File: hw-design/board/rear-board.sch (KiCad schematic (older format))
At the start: 20 parts, among them J1 CC_INPUT, J2 CC_OUTPUT, P7 CONN_01X16, P8 USB_OTG, P9 CONN_01X16, Q7 2N7002, Q8 2N7002, Q9 IRFML8244TRPBF

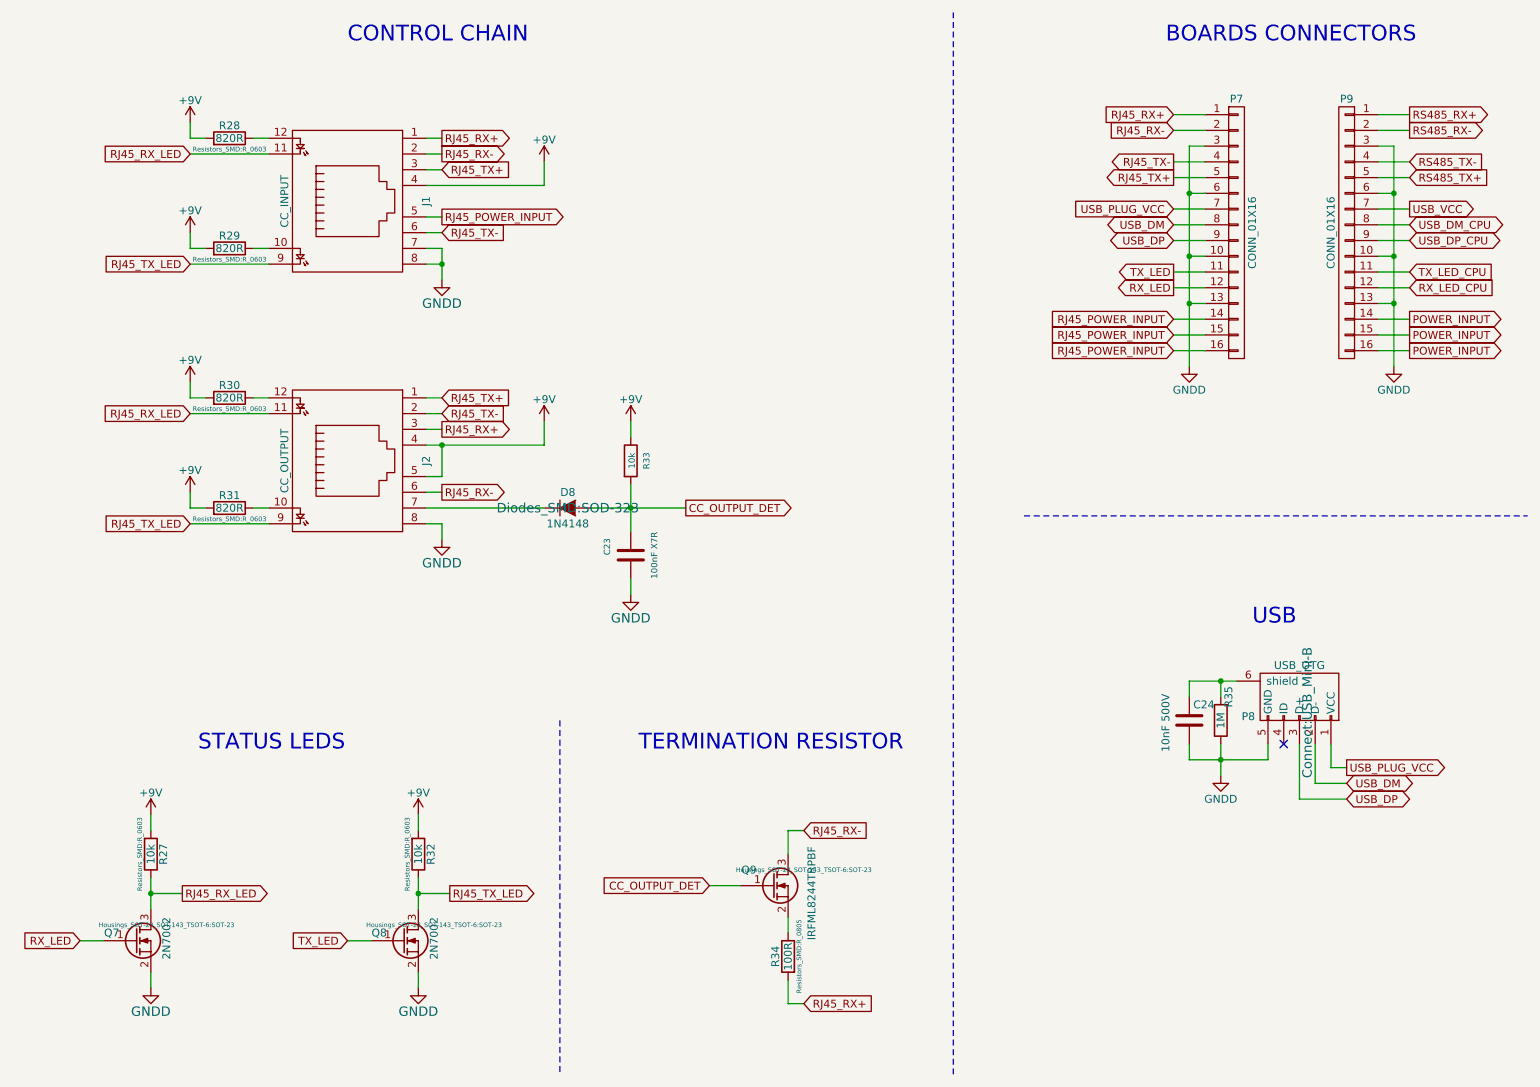
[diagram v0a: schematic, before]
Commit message: fix power voltage
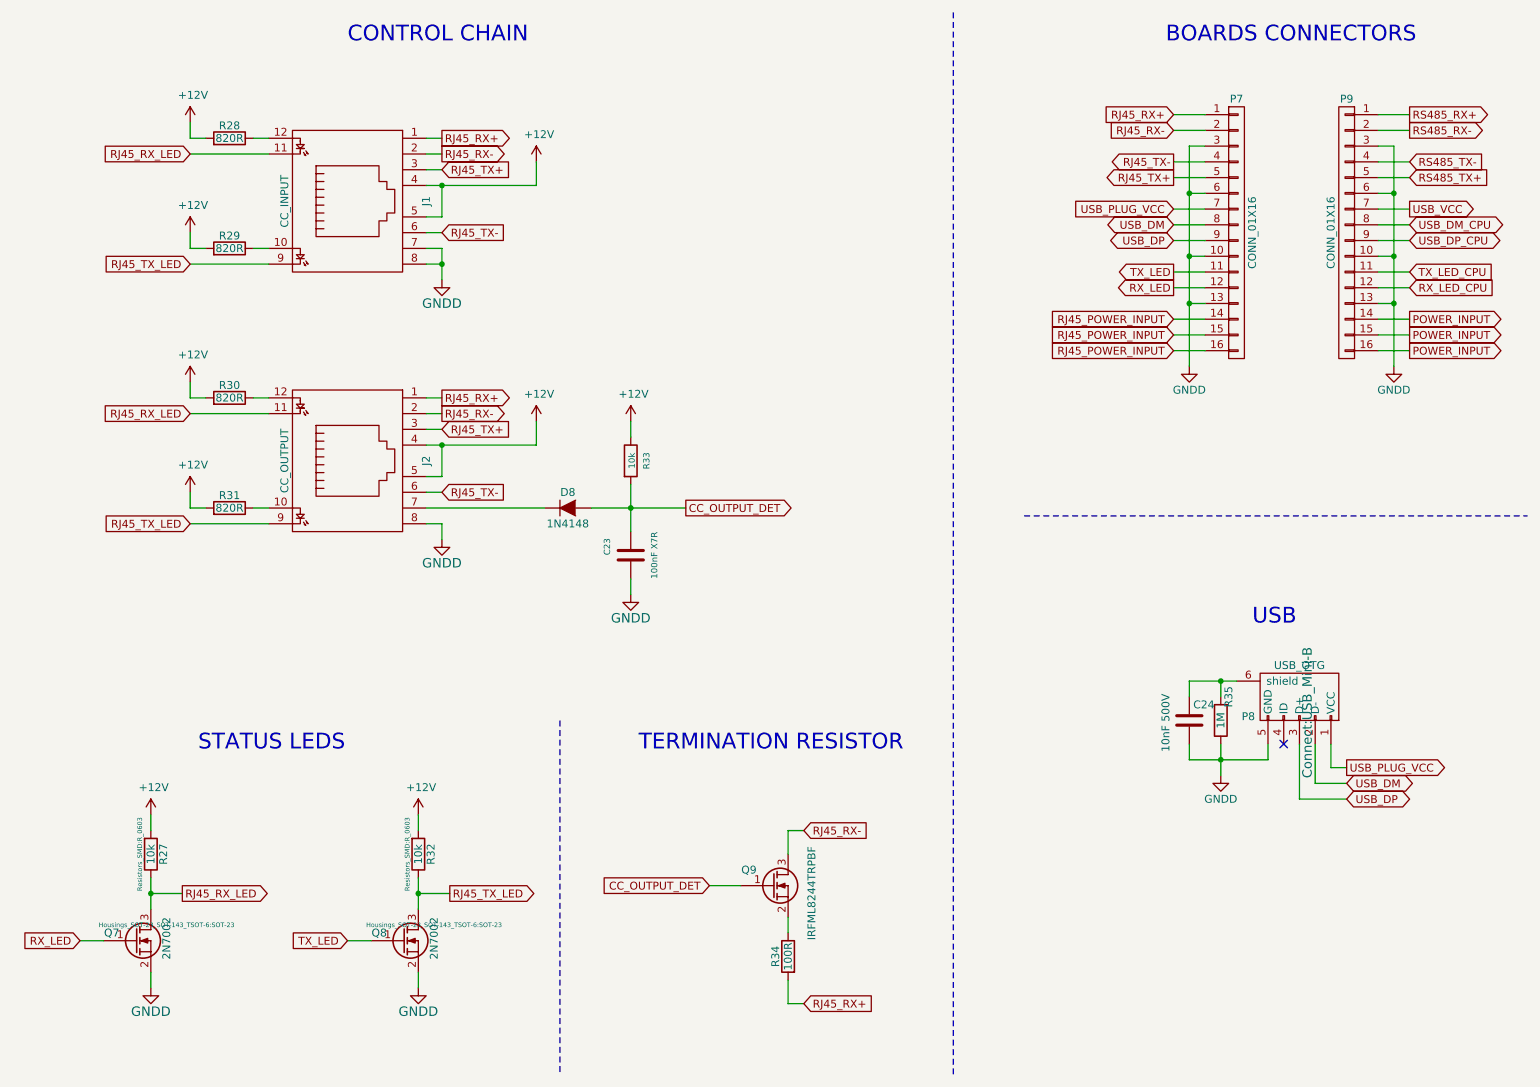
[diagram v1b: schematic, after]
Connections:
- net RJ45_POWER_INPUT: no longer J1.5
- net RJ45_RX+: now also J2.1; no longer J2.3
- net RJ45_RX-: now also J2.2; no longer J2.6
- net RJ45_TX+: now also J2.3; no longer J2.1
- net RJ45_TX-: now also J2.6; no longer J2.2
- net +9V renamed +12V
- net +12V: now also J1.5
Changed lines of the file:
@@
-$EndComp
-$Comp
-L +9V #PWR085
-U 1 1 55B26422
-P 4700 3300
-F 0 "#PWR085" H 4700 3150 50  0001 C CNN
-F 1 "+9V" H 4700 3440 50  0000 C CNN
-F 2 "" H 4700 3300 60  0000 C CNN
-F 3 "" H 4700 3300 60  0000 C CNN
-	1    4700 3300
-	1    0    0    -1
-$EndComp
-$Comp
-L +9V #PWR086
-U 1 1 55B26428
-P 4150 3300
-F 0 "#PWR086" H 4150 3150 50  0001 C CNN
-F 1 "+9V" H 4150 3440 50  0000 C CNN
-F 2 "" H 4150 3300 60  0000 C CNN
-F 3 "" H 4150 3300 60  0000 C CNN
-	1    4150 3300
-	1    0    0    -1
-$EndComp
-$Comp
-L +9V #PWR087
-U 1 1 55B2642E
-P 4150 1650
-F 0 "#PWR087" H 4150 1500 50  0001 C CNN
-F 1 "+9V" H 4150 1790 50  0000 C CNN
-F 2 "" H 4150 1650 60  0000 C CNN
-F 3 "" H 4150 1650 60  0000 C CNN
-	1    4150 1650
-	1    0    0    -1
 $EndComp
 $Comp
@@
 F 0 "D8" H 4300 3950 50  0000 C CNN
 F 1 "1N4148" H 4300 3750 50  0000 C CNN
-F 2 "Diodes_SMD:SOD-323" H 4300 3850 60  0000 C CNN
+F 2 "Diodes_SMD:SOD-323" H 4300 3850 60  0001 C CNN
 F 3 "" H 4300 3850 60  0000 C CNN
 F 4 "1N4148WX-TP" H -250 -250 50  0001 C CNN "MPN"
@@
 F 0 "R30" V 2230 3150 50  0000 C CNN
 F 1 "820R" V 2150 3150 50  0000 C CNN
-F 2 "Resistors_SMD:R_0603" V 2080 3150 30  0000 C CNN
+F 2 "Resistors_SMD:R_0603" V 2080 3150 30  0001 C CNN
 F 3 "" H 2150 3150 30  0000 C CNN
 F 4 "ESR03EZPJ821" H -250 -250 50  0001 C CNN "MPN"
@@
 F 0 "R28" V 2230 1500 50  0000 C CNN
 F 1 "820R" V 2150 1500 50  0000 C CNN
-F 2 "Resistors_SMD:R_0603" V 2080 1500 30  0000 C CNN
+F 2 "Resistors_SMD:R_0603" V 2080 1500 30  0001 C CNN
 F 3 "" H 2150 1500 30  0000 C CNN
 F 4 "ESR03EZPJ821" H -250 -100 50  0001 C CNN "MPN"
@@
 F 0 "R31" V 2230 3850 50  0000 C CNN
 F 1 "820R" V 2150 3850 50  0000 C CNN
-F 2 "Resistors_SMD:R_0603" V 2080 3850 30  0000 C CNN
+F 2 "Resistors_SMD:R_0603" V 2080 3850 30  0001 C CNN
 F 3 "" H 2150 3850 30  0000 C CNN
 F 4 "ESR03EZPJ821" H -250 -250 50  0001 C CNN "MPN"
@@
 F 0 "R29" V 2230 2200 50  0000 C CNN
 F 1 "820R" V 2150 2200 50  0000 C CNN
-F 2 "Resistors_SMD:R_0603" V 2080 2200 30  0000 C CNN
+F 2 "Resistors_SMD:R_0603" V 2080 2200 30  0001 C CNN
 F 3 "" H 2150 2200 30  0000 C CNN
 F 4 "ESR03EZPJ821" H -250 -100 50  0001 C CNN "MPN"
 	1    2150 2200
 	0    1    -1   0
-$EndComp
-$Comp
-L +9V #PWR088
-U 1 1 55B2645C
-P 1900 3050
-F 0 "#PWR088" H 1900 2900 50  0001 C CNN
-F 1 "+9V" H 1900 3190 50  0000 C CNN
-F 2 "" H 1900 3050 60  0000 C CNN
-F 3 "" H 1900 3050 60  0000 C CNN
-	1    1900 3050
-	1    0    0    -1
-$EndComp
-$Comp
-L +9V #PWR089
-U 1 1 55B26462
-P 1900 3750
-F 0 "#PWR089" H 1900 3600 50  0001 C CNN
-F 1 "+9V" H 1900 3890 50  0000 C CNN
-F 2 "" H 1900 3750 60  0000 C CNN
-F 3 "" H 1900 3750 60  0000 C CNN
-	1    1900 3750
-	1    0    0    -1
-$EndComp
-$Comp
-L +9V #PWR090
-U 1 1 55B26468
-P 1900 2100
-F 0 "#PWR090" H 1900 1950 50  0001 C CNN
-F 1 "+9V" H 1900 2240 50  0000 C CNN
-F 2 "" H 1900 2100 60  0000 C CNN
-F 3 "" H 1900 2100 60  0000 C CNN
-	1    1900 2100
-	1    0    0    -1
-$EndComp
-$Comp
-L +9V #PWR091
-U 1 1 55B2646E
-P 1900 1400
-F 0 "#PWR091" H 1900 1250 50  0001 C CNN
-F 1 "+9V" H 1900 1540 50  0000 C CNN
-F 2 "" H 1900 1400 60  0000 C CNN
-F 3 "" H 1900 1400 60  0000 C CNN
-	1    1900 1400
-	1    0    0    -1
 $EndComp
 Text GLabel 3500 1700 2    50   Input ~ 0
@@
 Text GLabel 3500 1600 2    50   Output ~ 0
 RJ45_RX-
-Text GLabel 3500 3150 2    50   Input ~ 0
+Text GLabel 3500 3350 2    50   Input ~ 0
 RJ45_TX+
-Text GLabel 3500 3250 2    50   Input ~ 0
+Text GLabel 3500 3750 2    50   Input ~ 0
 RJ45_TX-
-Text GLabel 3500 3350 2    50   Output ~ 0
+Text GLabel 3500 3150 2    50   Output ~ 0
 RJ45_RX+
-Text GLabel 3500 3750 2    50   Output ~ 0
+Text GLabel 3500 3250 2    50   Output ~ 0
 RJ45_RX-
-Text GLabel 3500 2000 2    50   Output ~ 0
-RJ45_POWER_INPUT
 Text GLabel 5050 3850 2    50   Output ~ 0
 CC_OUTPUT_DET
@@
 $EndComp
 $Comp
-L +9V #PWR094
-U 1 1 55B30E71
-P 1650 5800
-F 0 "#PWR094" H 1650 5650 50  0001 C CNN
-F 1 "+9V" H 1650 5940 50  0000 C CNN
-F 2 "" H 1650 5800 60  0000 C CNN
-F 3 "" H 1650 5800 60  0000 C CNN
-	1    1650 5800
-	1    0    0    -1
-$EndComp
-$Comp
 L Q_NMOS_GSD Q8
 U 1 1 55B30E78
@@
 	1    0    0    1
 $EndComp
-$Comp
-L +9V #PWR096
-U 1 1 55B30E8D
-P 3350 5800
-F 0 "#PWR096" H 3350 5650 50  0001 C CNN
-F 1 "+9V" H 3350 5940 50  0000 C CNN
-F 2 "" H 3350 5800 60  0000 C CNN
-F 3 "" H 3350 5800 60  0000 C CNN
-	1    3350 5800
-	1    0    0    -1
-$EndComp
 Text Notes 1950 5400 0    100  ~ 0
 STATUS LEDS
@@
 F 0 "Q9" H 5500 6350 50  0000 R CNN
 F 1 "IRFML8244TRPBF" V 5850 6500 50  0000 R CNN
-F 2 "Housings_SOT-23_SOT-143_TSOT-6:SOT-23" H 5800 6350 29  0000 C CNN
+F 2 "Housings_SOT-23_SOT-143_TSOT-6:SOT-23" H 5800 6350 29  0001 C CNN
 F 3 "" H 5600 6250 60  0000 C CNN
 F 4 "IRFML8244TRPBF" H -2600 1300 50  0001 C CNN "MPN"
@@
 F 0 "R34" V 5780 6700 50  0000 C CNN
 F 1 "100R" V 5700 6700 50  0000 C CNN
-F 2 "Resistors_SMD:R_0805" V 5630 6700 30  0000 C CNN
+F 2 "Resistors_SMD:R_0805" V 5630 6700 30  0001 C CNN
 F 3 "" H 5700 6700 30  0000 C CNN
 F 4 "ERJ-P06F1000V" H -2600 1300 50  0001 C CNN "MPN"
@@
 	4700 3400 4700 3300
 Wire Wire Line
-	3400 3450 4150 3450
-Wire Wire Line
-	4150 3450 4150 3300
+	3400 3450 4100 3450
 Wire Wire Line
 	3400 3650 3500 3650
@@
 	1900 1500 1900 1400
 Wire Wire Line
-	3400 1800 4150 1800
-Wire Wire Line
-	4150 1800 4150 1650
+	3400 1800 4100 1800
 Connection ~ 3500 2300
 Connection ~ 4700 3850
@@
 Wire Wire Line
 	9450 2850 9650 2850
+$Comp
+L +12V #PWR?
+U 1 1 575F20CD
+P 1900 1400
+F 0 "#PWR?" H 1900 1250 50  0001 C CNN
+F 1 "+12V" H 1918 1574 50  0000 C CNN
+F 2 "" H 1900 1400 60  0000 C CNN
+F 3 "" H 1900 1400 60  0000 C CNN
+	1    1900 1400
+	1    0    0    -1
+$EndComp
+$Comp
+L +12V #PWR?
+U 1 1 575F21C6
+P 1900 2100
+F 0 "#PWR?" H 1900 1950 50  0001 C CNN
+F 1 "+12V" H 1918 2274 50  0000 C CNN
+F 2 "" H 1900 2100 60  0000 C CNN
+F 3 "" H 1900 2100 60  0000 C CNN
+	1    1900 2100
+	1    0    0    -1
+$EndComp
+$Comp
+L +12V #PWR?
+U 1 1 575F2249
+P 4100 1650
+F 0 "#PWR?" H 4100 1500 50  0001 C CNN
+F 1 "+12V" H 4118 1824 50  0000 C CNN
+F 2 "" H 4100 1650 60  0000 C CNN
+F 3 "" H 4100 1650 60  0000 C CNN
+	1    4100 1650
+	1    0    0    -1
+$EndComp
+$Comp
+L +12V #PWR?
+U 1 1 575F236C
+P 1900 3050
+F 0 "#PWR?" H 1900 2900 50  0001 C CNN
+F 1 "+12V" H 1918 3224 50  0000 C CNN
+F 2 "" H 1900 3050 60  0000 C CNN
+F 3 "" H 1900 3050 60  0000 C CNN
+	1    1900 3050
+	1    0    0    -1
+$EndComp
+$Comp
+L +12V #PWR?
+U 1 1 575F23B3
+P 1900 3750
+F 0 "#PWR?" H 1900 3600 50  0001 C CNN
+F 1 "+12V" H 1918 3924 50  0000 C CNN
+F 2 "" H 1900 3750 60  0000 C CNN
+F 3 "" H 1900 3750 60  0000 C CNN
+	1    1900 3750
+	1    0    0    -1
+$EndComp
+$Comp
+L +12V #PWR?
+U 1 1 575F23FA
+P 4700 3300
+F 0 "#PWR?" H 4700 3150 50  0001 C CNN
+F 1 "+12V" H 4718 3474 50  0000 C CNN
+F 2 "" H 4700 3300 60  0000 C CNN
+F 3 "" H 4700 3300 60  0000 C CNN
+	1    4700 3300
+	1    0    0    -1
+$EndComp
+$Comp
+L +12V #PWR?
+U 1 1 575F2441
+P 4100 3300
+F 0 "#PWR?" H 4100 3150 50  0001 C CNN
+F 1 "+12V" H 4118 3474 50  0000 C CNN
+F 2 "" H 4100 3300 60  0000 C CNN
+F 3 "" H 4100 3300 60  0000 C CNN
+	1    4100 3300
+	1    0    0    -1
+$EndComp
+Wire Wire Line
+	4100 3450 4100 3300
+Wire Wire Line
+	4100 1800 4100 1650
+Wire Wire Line
+	3500 2000 3500 1800
+Connection ~ 3500 1800
+$Comp
+L +12V #PWR?
+U 1 1 575F61FF
+P 1650 5800
+F 0 "#PWR?" H 1650 5650 50  0001 C CNN
+F 1 "+12V" H 1668 5974 50  0000 C CNN
+F 2 "" H 1650 5800 60  0000 C CNN
+F 3 "" H 1650 5800 60  0000 C CNN
+	1    1650 5800
+	1    0    0    -1
+$EndComp
+$Comp
+L +12V #PWR?
+U 1 1 575F6219
+P 3350 5800
+F 0 "#PWR?" H 3350 5650 50  0001 C CNN
+F 1 "+12V" H 3368 5974 50  0000 C CNN
+F 2 "" H 3350 5800 60  0000 C CNN
+F 3 "" H 3350 5800 60  0000 C CNN
+	1    3350 5800
+	1    0    0    -1
+$EndComp
 $EndSCHEMATC
